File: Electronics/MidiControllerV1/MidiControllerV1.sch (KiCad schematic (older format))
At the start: 47 parts

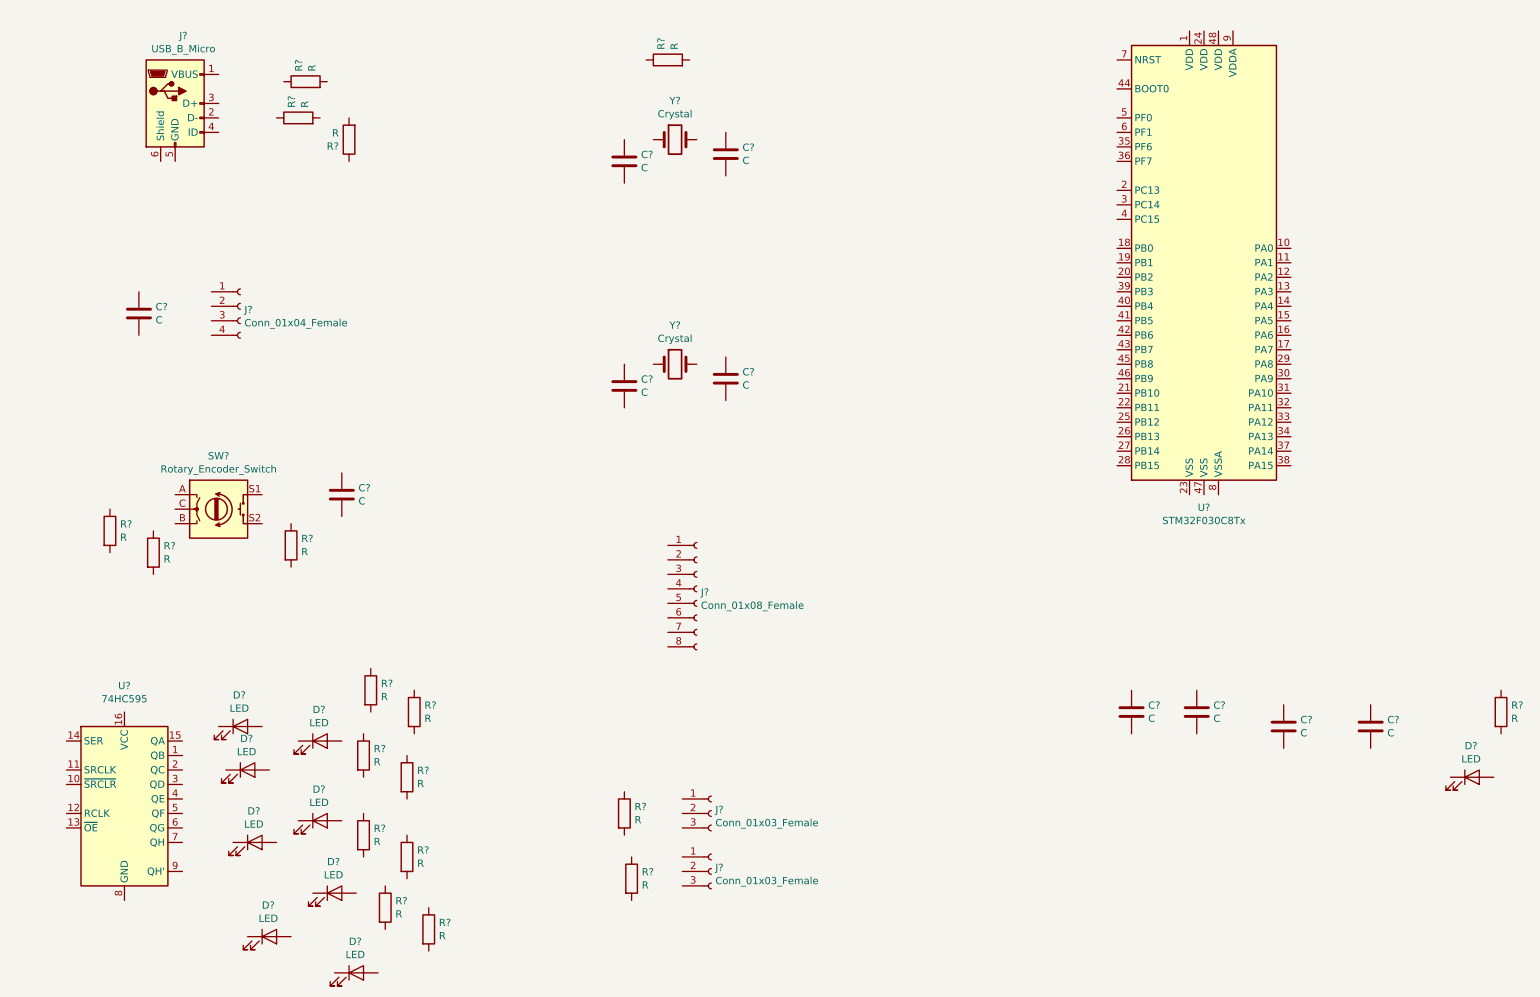
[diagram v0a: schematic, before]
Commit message: #2 Schematic wired up
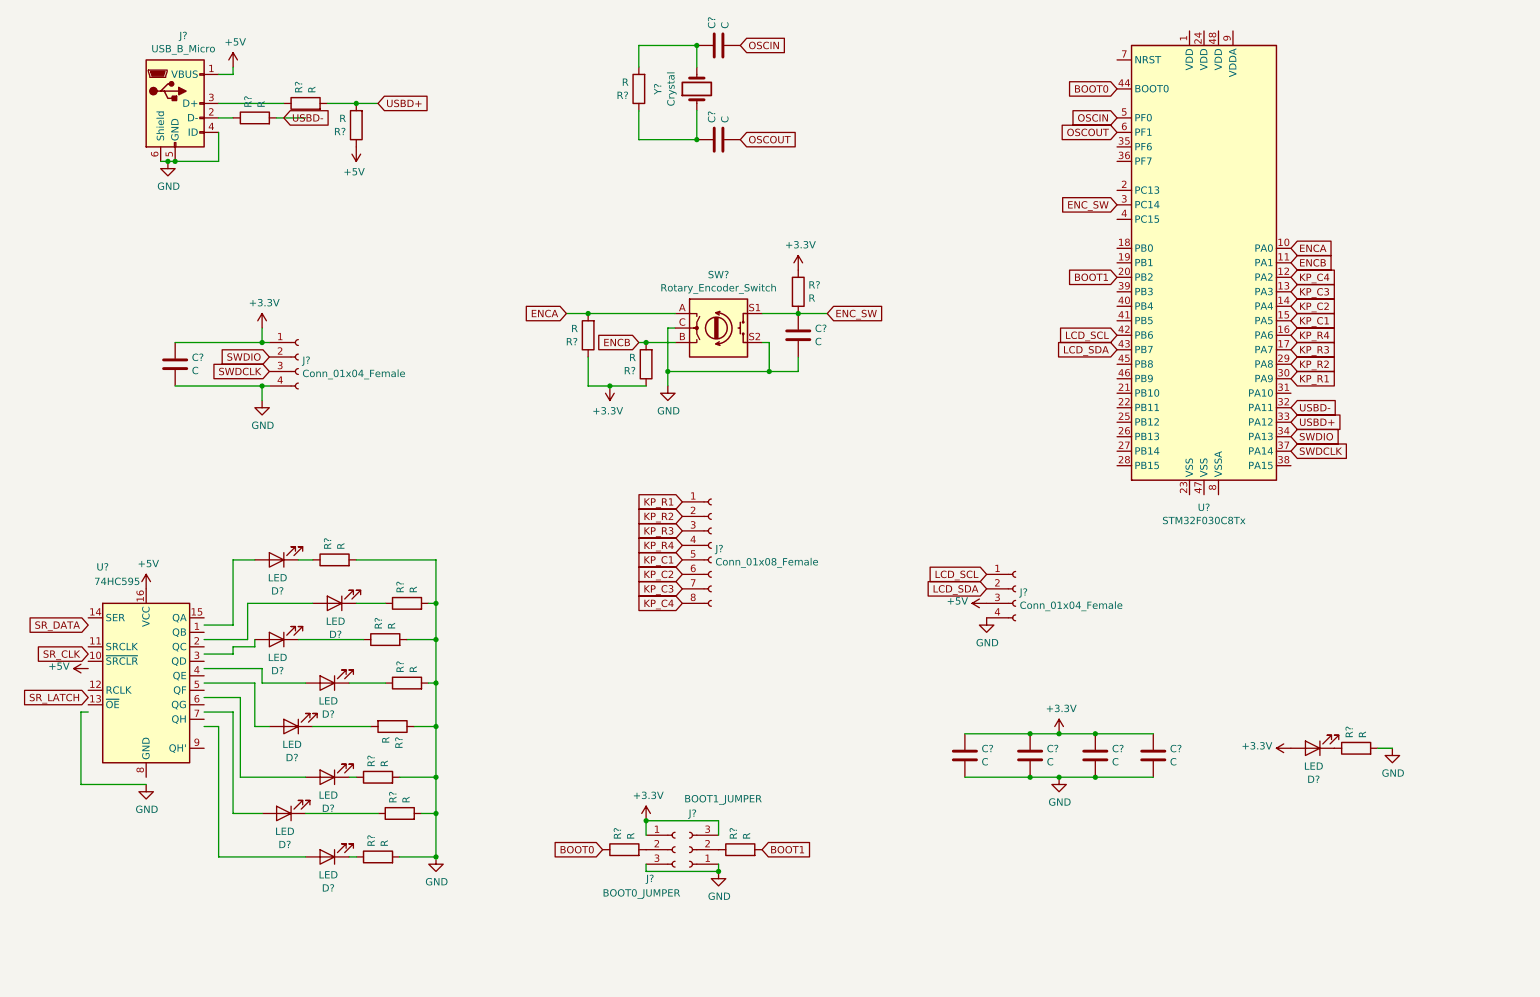
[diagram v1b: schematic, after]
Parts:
- removed C? (x2): C, symbol Device:C
- removed Y?: Crystal, symbol Device:Crystal
- added J?: Conn_01x04_Female, symbol Connector:Conn_01x04_Female
- J?: value Conn_01x03_Female -> BOOT1_JUMPER
- J?: value Conn_01x03_Female -> BOOT0_JUMPER
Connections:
- net labels added: +3.3V, +5V, BOOT0, BOOT1, ENCA, ENCB, ENC_SW, GND, KP_C1, KP_C2, KP_C3, KP_C4, KP_R1, KP_R2, KP_R3, KP_R4, LCD_SCL, LCD_SDA, OSCIN, OSCOUT, SR_CLK, SR_DATA, SR_LATCH, SWDCLK, SWDIO, USBD+, USBD-
- wire segments 0 -> 106
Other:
- moved on the sheet: C?, D?, J?, R?, SW?, U?, Y?
